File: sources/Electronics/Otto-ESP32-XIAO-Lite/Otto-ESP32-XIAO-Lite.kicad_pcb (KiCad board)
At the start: 2 copper layers, 60 x 52 mm, 53 parts, among them J1 Conn_01x03, J10 Conn_01x02, J12 OLED 0,91" - I2C (SKU21796), J13 MPU6050, J2 Conn_01x03, J3 Conn_01x03, J4 Conn_01x03, J5 Conn_01x03, J6 Conn_01x03, J7 Ultrasonic sensor, J8 PCA9685, SW1 SW_SPDT, U1 MOUDLE-SEEEDUINO-XIAO-ESP32C3, U2 R-78E5.0-1.0

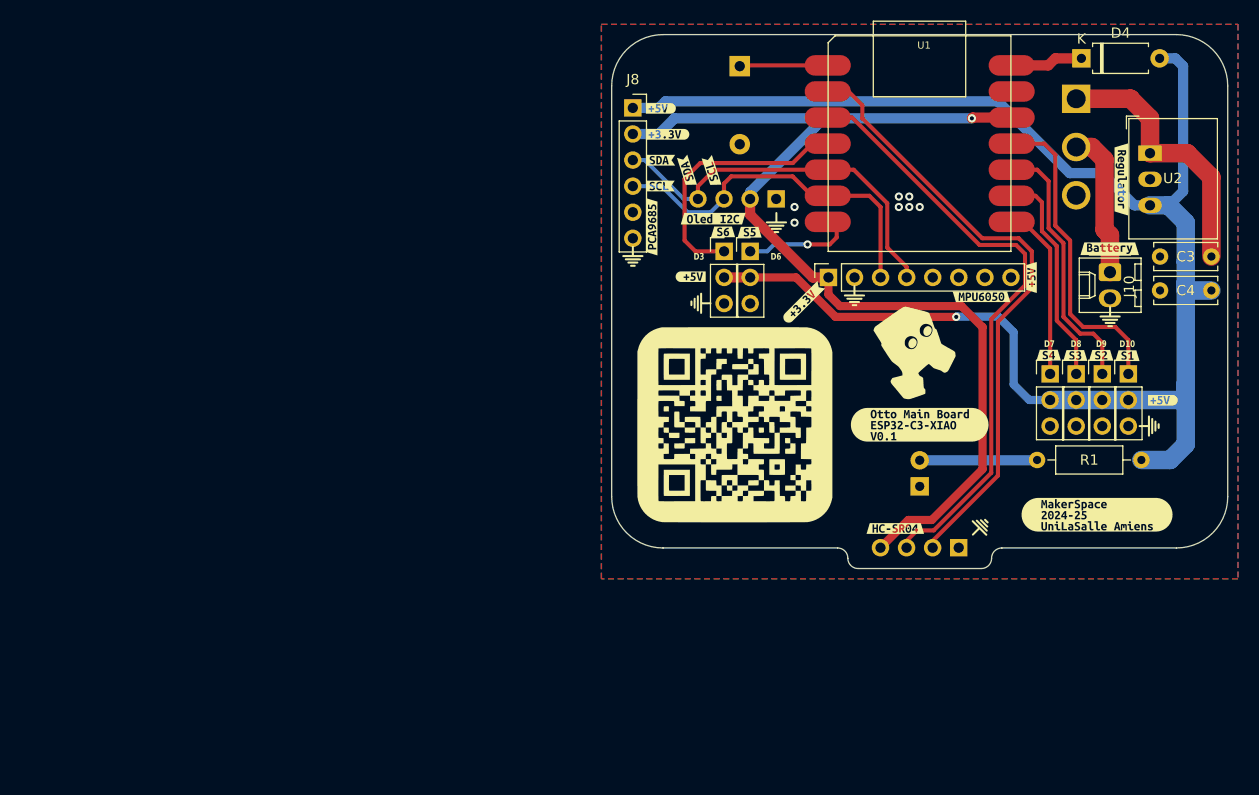
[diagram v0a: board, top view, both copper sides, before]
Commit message: update documentation
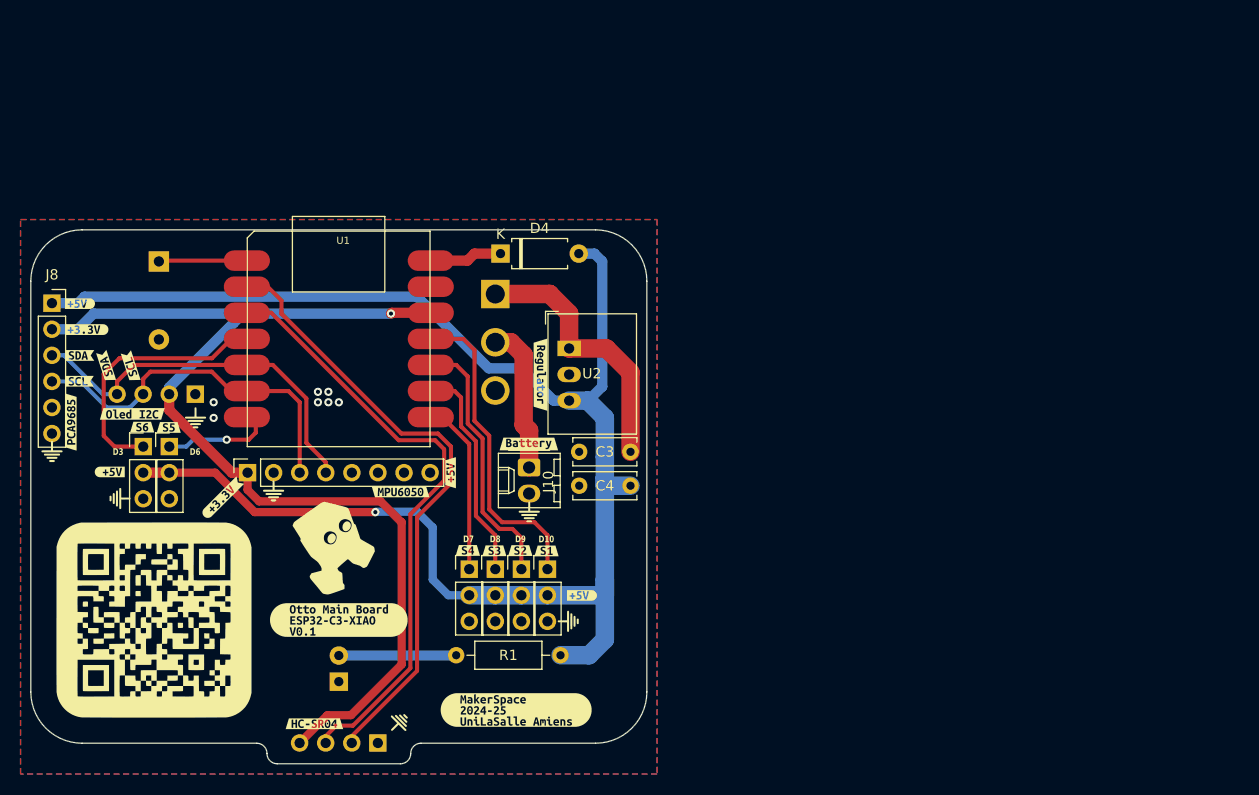
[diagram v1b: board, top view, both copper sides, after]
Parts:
- moved kibuzzard-66E45B15 59.7 mm to (84.3, 92.7)
- moved kibuzzard-6707C6B3 59.7 mm to (93.1, 83.1)
- moved D1 59.7 mm to (73.4, 113.0)
- moved G*** 59.7 mm to (95.8, 107.1)
- moved G*** 59.7 mm to (67.1, 94.5)
- moved G*** 59.7 mm to (79.3, 117.0)
- moved J6 59.7 mm to (54.4, 90.1)
- moved J7 59.7 mm to (77.2, 119.0)
- moved J8 59.7 mm to (45.5, 76.2)
- moved kibuzzard-66E45B51 59.7 mm to (93.7, 100.3)
- moved kibuzzard-66E45BAB 59.7 mm to (48.2, 76.2)
- moved kibuzzard-6707CF99 59.7 mm to (73.4, 107.0)
- moved kibuzzard-67654523 59.7 mm to (53.2, 82.3)
- moved G*** 59.7 mm to (55.4, 107.0)
- moved J12 59.7 mm to (59.4, 85.0)
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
